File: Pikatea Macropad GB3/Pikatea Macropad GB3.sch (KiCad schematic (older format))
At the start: 29 parts, among them J1 AVR-ISP-6, J2 USB_B_Mini, J3 Conn_01x03_Male, J4 Conn_01x03_Male, J5 Conn_01x03_Male, J6 Conn_01x06_Male, J7 Conn_01x03_Male, SW1 SW_DPST, SW2 Rotary_Encoder_Switch, U1 ATMEGA32U4-EP, X1 16MHz

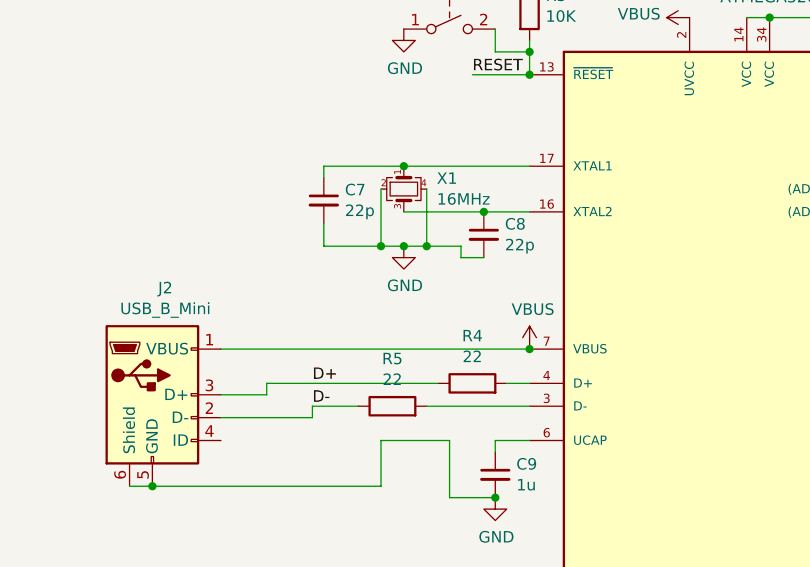
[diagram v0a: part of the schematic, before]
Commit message: start finngus project
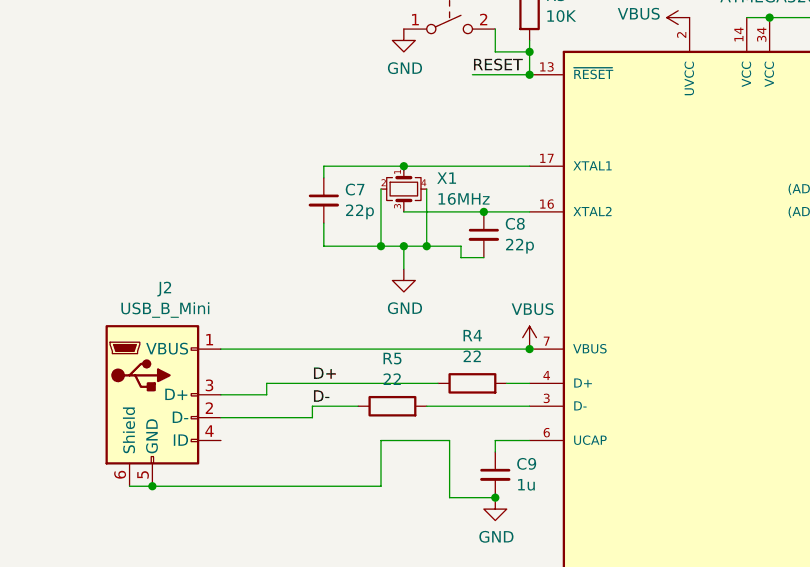
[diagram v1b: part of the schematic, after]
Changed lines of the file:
@@
 L power:GND #PWR0106
 U 1 1 5FC36DC8
-P 5400 3800
-F 0 "#PWR0106" H 5400 3550 50  0001 C CNN
-F 1 "GND" H 5405 3627 50  0000 C CNN
-F 2 "" H 5400 3800 50  0001 C CNN
-F 3 "" H 5400 3800 50  0001 C CNN
-	1    5400 3800
+P 5400 3900
+F 0 "#PWR0106" H 5400 3650 50  0001 C CNN
+F 1 "GND" H 5405 3727 50  0000 C CNN
+F 2 "" H 5400 3900 50  0001 C CNN
+F 3 "" H 5400 3900 50  0001 C CNN
+	1    5400 3900
 	1    0    0    -1
 $EndComp
@@
 Text Label 5750 2200 0    50   ~ 0
 D1
+Wire Wire Line
+	5400 3800 5400 3900
 $EndSCHEMATC
